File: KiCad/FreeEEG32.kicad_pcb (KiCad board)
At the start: 4 copper layers, 70 x 70 mm, 177 parts, among them P1 CONN_02X10, P11 CONN_01X03, P2 CONN_02X10, P3 CONN_02X10, P4 CONN_02X10, P6 CONN_02X03, P7 CONN_02X03, P8 USB_B, SW1 NRST, SW2 SWITCH_INV, SW3 SWITCH_INV, T1 da2303, U1 ADP7118AUJZ-3.3_TSOT, U10 TPD4E1B06, U11 TPD4E1B06, U12 MPU-6500, U13 AD7770, U14 ADR4525, U15 TPD4E1B06, U16 TPD4E1B06, U17 TPD4E1B06, U18 TPD4E1B06, U19 TLV73333PDBVT, U2 ADP7118AUJZ-3.3_TSOT, U20 AD7770, U21 ADR4525, U22 TPD4E1B06, U23 TPD4E1B06, U24 TPD4E1B06, U25 TPD4E1B06, U27 AD7770, U28 ADR4525, U29 TPD4E1B06, U3 8.192MHz, U30 TPD4E1B06, U31 TPD4E1B06, U32 TPD4E1B06, U34 AD7770, U35 ADUM1402BRWZ, U36 ISO7341c_spi, U37 STM32F427ZI_4side_short, U39 ADP7118AUJZ-3.3_TSOT, U40 CP2102N-24, U43 473521001, U5 ESP-12F, U6 SN6505A, U7 ADR4525, U8 TPD4E1B06, U9 TPD4E1B06, Y2 8MHz

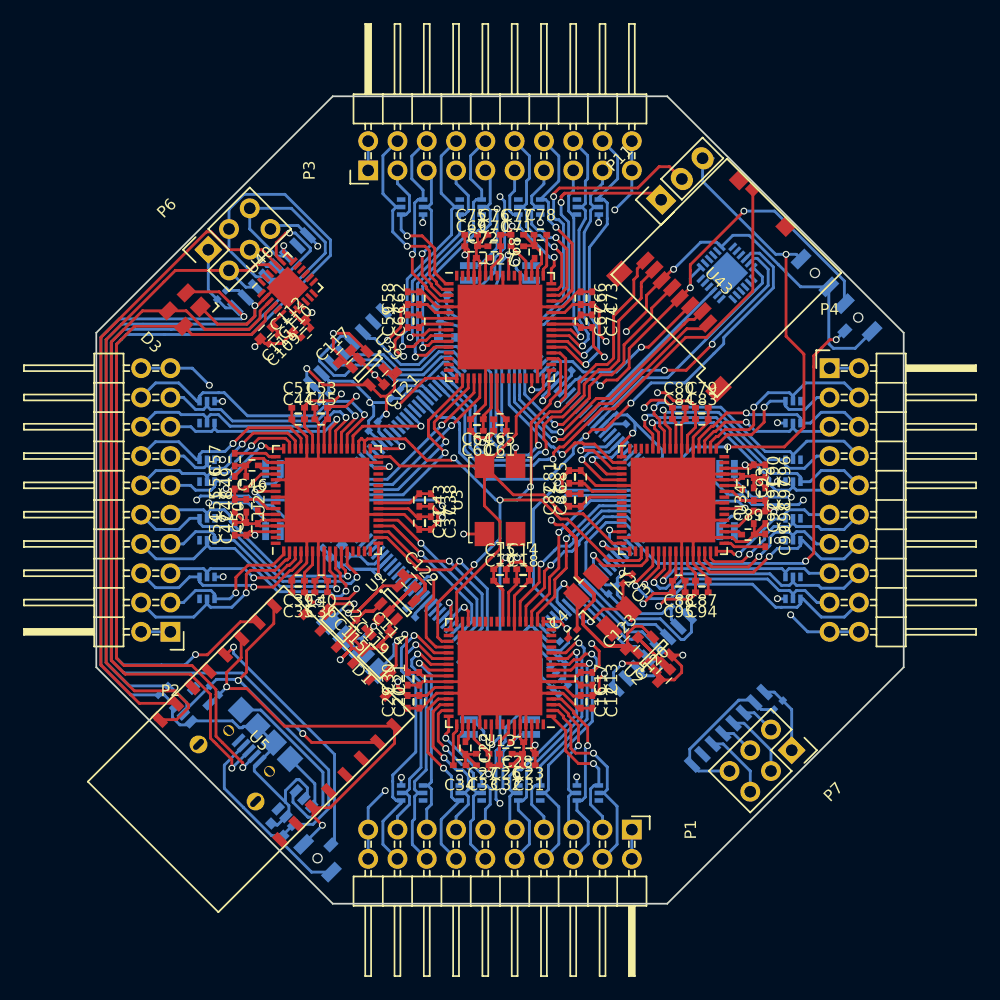
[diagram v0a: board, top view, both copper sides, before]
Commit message: kicad
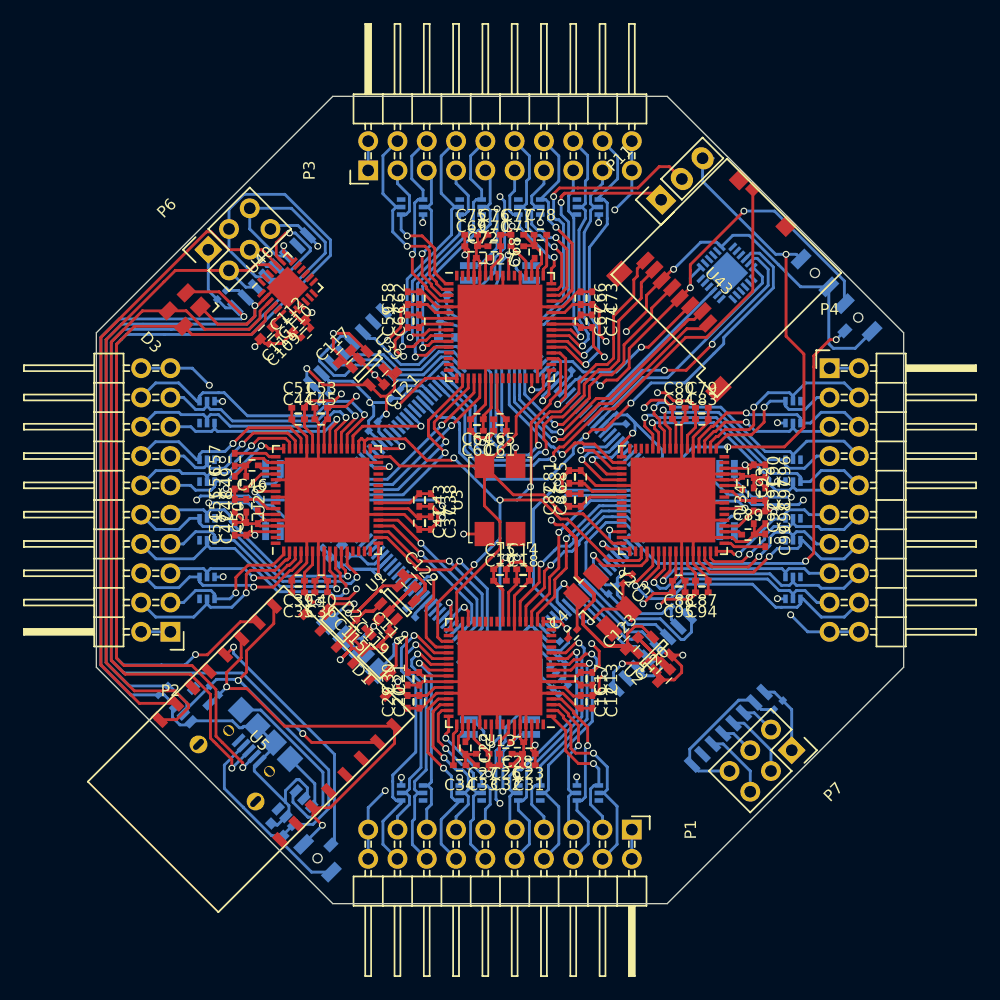
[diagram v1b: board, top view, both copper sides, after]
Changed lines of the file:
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@@
     (links 734)
     (no_connects 27)
-    (area -35.075001 -35.075001 35.075001 35.075001)
+    (area -35.005001 -35.005001 35.005001 35.005001)
     (thickness 1.6)
-    (drawings 47)
+    (drawings 39)
     (tracks 3168)
     (zones 0)
@@
     (trace_min 0.2)
     (segment_width 0.2)
-    (edge_width 0.15)
+    (edge_width 0.001)
     (via_size 0.6)
     (via_drill 0.4)
@@
     (pad "" np_thru_hole circle (at 0 0 315) (size 0.8 0.8) (drill 0.8) (layers *.Cu *.Mask))
   )
+  (gr_line (start -14.49746 -34.99746) (end -34.99746 -14.49746) (angle 90) (layer Edge.Cuts) (width 0.001))
+  (gr_line (start 14.5 -34.99746) (end -14.5 -34.99746) (angle 90) (layer Edge.Cuts) (width 0.001))
   (gr_line (start 0 0) (end 35 0) (angle 90) (layer Cmts.User) (width 0.2))
   (gr_line (start 0 0) (end -34.925 0) (angle 90) (layer Cmts.User) (width 0.2))
@@
   (gr_line (start 0 0) (end 24.765 -24.765) (angle 90) (layer Cmts.User) (width 0.2))
   (gr_circle (center 0 0) (end 2 50) (layer Dwgs.User) (width 0.2))
-  (gr_line (start 14.5 35) (end 35 14.5) (angle 90) (layer Edge.Cuts) (width 0.15))
-  (gr_line (start -14.5 35) (end 14.5 35) (angle 90) (layer Edge.Cuts) (width 0.15))
-  (gr_line (start -35 14.5) (end -14.5 35) (angle 90) (layer Edge.Cuts) (width 0.15))
-  (gr_line (start -35 -14.5) (end -35 14.5) (angle 90) (layer Edge.Cuts) (width 0.15))
-  (gr_line (start -14.5 -35) (end -35 -14.5) (angle 90) (layer Edge.Cuts) (width 0.15))
-  (gr_line (start 14.5 -35) (end -14.5 -35) (angle 90) (layer Edge.Cuts) (width 0.15))
-  (gr_line (start 35 -14.5) (end 14.5 -35) (angle 90) (layer Edge.Cuts) (width 0.15))
-  (gr_line (start 35 14.5) (end 35 -14.5) (angle 90) (layer Edge.Cuts) (width 0.15))
+  (gr_line (start 14.49746 34.99746) (end 34.99746 14.49746) (angle 90) (layer Edge.Cuts) (width 0.001))
+  (gr_line (start -14.5 34.99746) (end 14.5 34.99746) (angle 90) (layer Edge.Cuts) (width 0.001))
+  (gr_line (start -34.99746 14.49746) (end -14.49746 34.99746) (angle 90) (layer Edge.Cuts) (width 0.001))
+  (gr_line (start -34.99746 -14.5) (end -34.99746 14.5) (angle 90) (layer Edge.Cuts) (width 0.001))
+  (gr_line (start 34.99746 -14.49746) (end 14.49746 -34.99746) (angle 90) (layer Edge.Cuts) (width 0.001))
+  (gr_line (start 34.99746 14.5) (end 34.99746 -14.5) (angle 90) (layer Edge.Cuts) (width 0.001))
   (gr_circle (center 0 0) (end 2.54 -19.05) (layer Dwgs.User) (width 0.2))
   (gr_circle (center 0 0) (end 0 -8.89) (layer Dwgs.User) (width 0.2))
@@
   (gr_line (start 0 0) (end 0 -35) (angle 90) (layer Cmts.User) (width 0.2))
   (target plus (at 0 0) (size 5) (width 0.15) (layer Edge.Cuts))
-  (gr_line (start -35 -15) (end -15 -35) (angle 90) (layer Cmts.User) (width 0.2))
-  (gr_line (start -35 15) (end -35 -15) (angle 90) (layer Cmts.User) (width 0.2))
-  (gr_line (start -15 35) (end -35 15) (angle 90) (layer Cmts.User) (width 0.2))
-  (gr_line (start 15 35) (end -15 35) (angle 90) (layer Cmts.User) (width 0.2))
-  (gr_line (start 35 15) (end 15 35) (angle 90) (layer Cmts.User) (width 0.2))
-  (gr_line (start 35 -15) (end 35 15) (angle 90) (layer Cmts.User) (width 0.2))
-  (gr_line (start 15 -35) (end 35 -15) (angle 90) (layer Cmts.User) (width 0.2))
-  (gr_line (start -15 -35) (end 15 -35) (angle 90) (layer Cmts.User) (width 0.2))
   (gr_line (start 35 -35) (end -35 -35) (angle 90) (layer Dwgs.User) (width 0.2))
   (gr_line (start 35 35) (end 35 -35) (angle 90) (layer Dwgs.User) (width 0.2))
